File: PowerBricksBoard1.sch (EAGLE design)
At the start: 16 parts

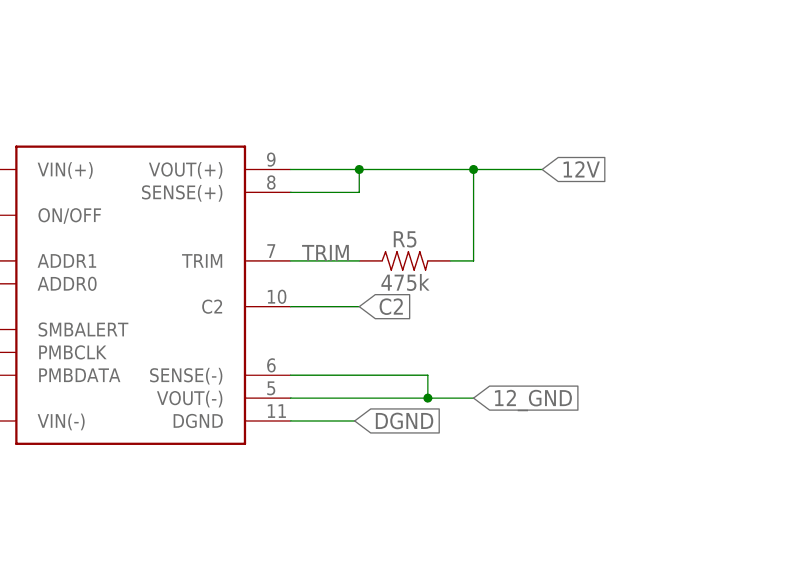
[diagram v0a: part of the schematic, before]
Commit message: Revert "Revert "trim""
This reverts commit 46b5d4a1c2a012013371b894087438f3b54206c6.
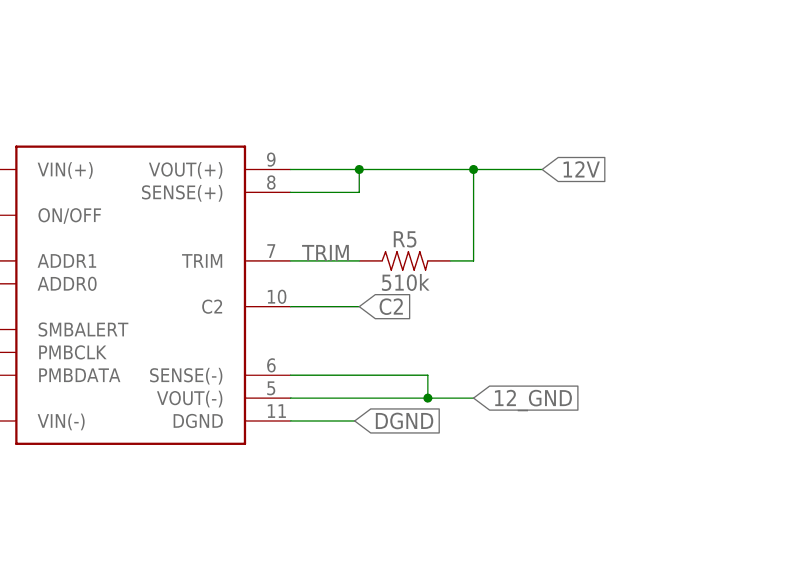
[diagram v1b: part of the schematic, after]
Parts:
- R5: value 475k -> 510k
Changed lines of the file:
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@@
 <part name="R4" library="SparkFun-Resistors" library_urn="urn:adsk.eagle:library:532" deviceset="RESISTOR" device="0603" package3d_urn="urn:adsk.eagle:package:39650/1" value=" "/>
 <part name="R3" library="SparkFun-Resistors" library_urn="urn:adsk.eagle:library:532" deviceset="RESISTOR" device="0603" package3d_urn="urn:adsk.eagle:package:39650/1" value=" "/>
-<part name="R5" library="SparkFun-Resistors" library_urn="urn:adsk.eagle:library:532" deviceset="RESISTOR" device="0603" package3d_urn="urn:adsk.eagle:package:39650/1" value="475k"/>
+<part name="R5" library="SparkFun-Resistors" library_urn="urn:adsk.eagle:library:532" deviceset="RESISTOR" device="0603" package3d_urn="urn:adsk.eagle:package:39650/1" value="510k"/>
 <part name="U$1" library="Brick_Dist_Connector" deviceset="BRICK2DIST" device=""/>
 </parts>
